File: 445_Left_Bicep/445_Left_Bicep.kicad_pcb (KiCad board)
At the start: 2 copper layers, 60.1 x 48.6 mm, 5 parts, among them J1 69167-114HLF, J2 SM02B-SRSS-TB_LF__SN_, U1 ESP32-WROOM-32, U2 LSM6DSMTR, U3 LP2950CZ-3.3_LFT3

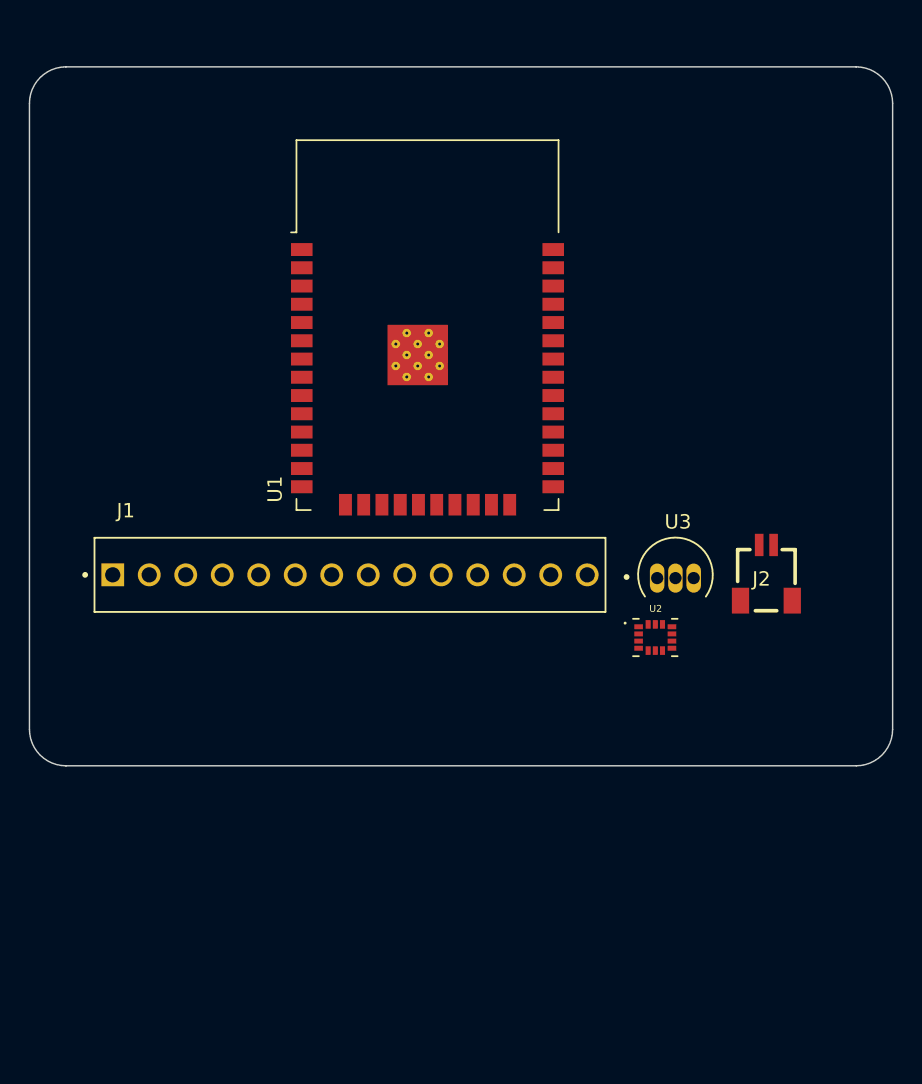
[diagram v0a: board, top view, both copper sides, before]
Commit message: Layout First Draft
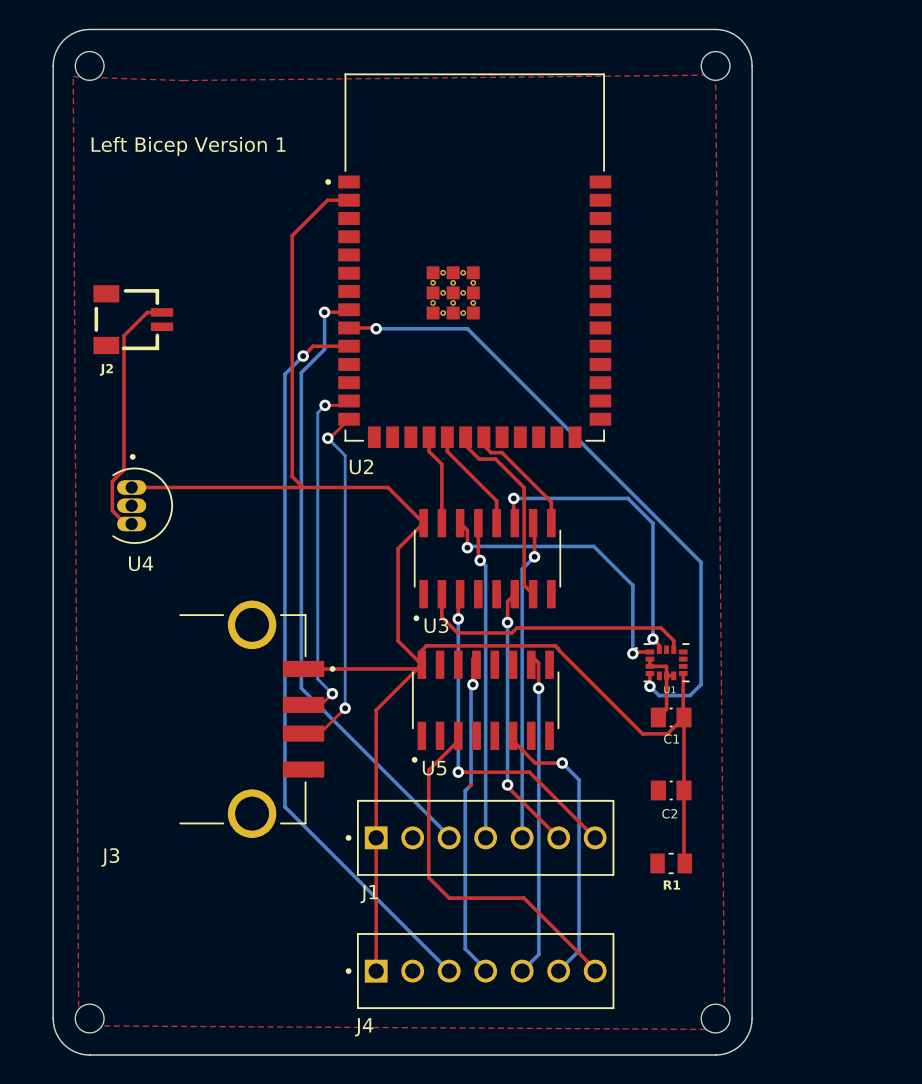
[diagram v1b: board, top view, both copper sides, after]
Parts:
- added C1: 100nF, CL21F104ZAANNNC:CAPC2012X135N, F.Cu at (150.6, 112.0)
- added C2: 100nF, CL21F104ZAANNNC:CAPC2012X135N, F.Cu at (150.6, 117.1)
- added H1: MountingHole, MountingHole:MountingHole_2mm, F.Cu at (110.1, 66.7)
- added H2: MountingHole, MountingHole:MountingHole_2mm, F.Cu at (153.7, 66.7)
- added H3: MountingHole, MountingHole:MountingHole_2mm, F.Cu at (110.1, 133.0)
- added H4: MountingHole, MountingHole:MountingHole_2mm, F.Cu at (153.7, 133.0)
- added J3: 87583-2010RPLF, 87583-2010RPLF:AMPHENOL_87583-2010RPLF, F.Cu at (121.4, 112.1)
- added J4: 69167-107HLF, 69167-107HLF:AMPHENOL_69167-107HLF, F.Cu at (137.7, 129.7)
- added R1: 10k, RMCF0805JG10K0:RESC2012X65N, F.Cu at (150.6, 122.2)
- added U4: LP2950CZ-3.3_LFT3, LP2950CZ-3.3_LFT3:TO92127P521H735-3, F.Cu at (113.8, 97.3)
- added U5: TS3A5018D, TS3A5018D:SOIC127P600X175-16N, F.Cu at (137.7, 110.8)
- J1: value 69167-114HLF -> 69167-107HLF; footprint 69167-114HLF:AMPHENOL_69167-114HLF -> 69167-107HLF:AMPHENOL_69167-107HLF
- U1: value ESP32-WROOM-32 -> LSM6DSMTR; footprint RF_Module:ESP32-WROOM-32 -> LSM6DSMTR (1):PQFN50P300X250X86-14N
- U2: value LSM6DSMTR -> ESP32-S3-WROOM-1-N16R8; footprint LSM6DSMTR (1):PQFN50P300X250X86-14N -> ESP32-S3-WROOM-1-N16R8:XCVR_ESP32-S3-WROOM-1-N16R8
- U3: value LP2950CZ-3.3_LFT3 -> TS3A5018D; footprint LP2950CZ-3.3_LFT3:TO92127P521H735-3 -> TS3A5018D:SOIC127P600X175-16N
- moved J2 47.4 mm to (113.2, 84.3), turned to -90 degrees
- moved U2 29.3 mm to (136.9, 80.0)
- moved U1 26.4 mm to (150.3, 108.2)
- moved J1 20.6 mm to (137.7, 120.4)
- moved U3 13.1 mm to (137.8, 101.0), turned to 90 degrees
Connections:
- J1 pad 03: unconnected-(J1-Pad03) -> INT1_1
- J1 pad 04: MISO -> MISO_1
- J1 pad 05: MOSI -> MOSI_1
- J1 pad 06: CLK -> CLK1
- J1 pad 07: CS2 -> SENSOR_1
- J2 pad 1: Net-(U3-IN) -> /3.7V
- U1 pad 1: GND -> MISO_2
- U1 pad 12: unconnected-(U1-IO27-Pad12) -> SENSOR_2
- U1 pad 13: unconnected-(U1-IO14-Pad13) -> CLK2
- U1 pad 14: unconnected-(U1-IO12-Pad14) -> MOSI_2
- U1 pad 2: 3.3V -> GND
- U1 pad 3: unconnected-(U1-EN-Pad3) -> GND
- U1 pad 4: unconnected-(U1-SENSOR_VP-Pad4) -> INT1_2
- U1 pad 5: unconnected-(U1-SENSOR_VN-Pad5) -> +3.3V
- U1 pad 6: unconnected-(U1-IO34-Pad6) -> GND
- U1 pad 7: unconnected-(U1-IO35-Pad7) -> GND
- U1 pad 8: unconnected-(U1-IO32-Pad8) -> +3.3V
- U2 pad 1: MISO -> GND
- U2 pad 10: unconnected-(U2-OCS_AUX-Pad10) -> INT1_3
- U2 pad 12: CS1 -> Net-(BZ1-+)
- U2 pad 13: CLK -> D-
- U2 pad 14: MOSI -> D+
- U2 pad 2: GND -> +3.3V
- U2 pad 3: GND -> +3.3V
- U2 pad 6: GND -> unconnected-(U2-IO6-Pad6)
- U2 pad 7: GND -> unconnected-(U2-IO7-Pad7)
- U2 pad 8: +3.3V -> INT1_1
- U2 pad 9: unconnected-(U2-INT2/DEN/MDRDY-Pad9) -> INT1_2
- U3 pad 1: 3.3V -> SENSOR_SEL
- U3 pad 2: GND -> SENSOR_2
- U3 pad 3: Net-(U3-IN) -> SENSOR_1
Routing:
- net +3.3V: track 0.00 -> 123.1 mm
- net INT1_3: track 0.00 -> 51.7 mm, vias 0 -> 1
- net INT1_2: track 0.00 -> 44.8 mm, vias 0 -> 2
- net INT1_1: track 0.00 -> 43.3 mm, vias 0 -> 1
- net SENSOR_3: track 0.00 -> 25.7 mm
- net D+: track 0.00 -> 24.9 mm, vias 0 -> 2
- net D-: track 0.00 -> 24.8 mm, vias 0 -> 2
- net SENSOR_1: track 0.00 -> 23.9 mm, vias 0 -> 2
- net MISO_3: track 0.00 -> 23.0 mm, vias 0 -> 1
- net MOSI_3: track 0.00 -> 22.7 mm, vias 0 -> 1
- net MOSI_1: track 0.00 -> 22.3 mm, vias 0 -> 1
- net MISO_1: track 0.00 -> 22.1 mm, vias 0 -> 1
- net MOSI_2: track 0.00 -> 21.1 mm, vias 0 -> 2
- net CLK3: track 0.00 -> 20.6 mm, vias 0 -> 1
- net MISO_2: track 0.00 -> 20.4 mm, vias 0 -> 2
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- added copper zone on F.Cu, net GND
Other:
- board size 60.1 x 48.6 mm -> 48.6 x 71.4 mm
- board text added: "J2"
- board text added: "Left Bicep Version 1"
